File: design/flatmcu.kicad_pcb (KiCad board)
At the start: 4 copper layers, 77.8 x 63.2 mm, 127 parts, among them J1 Hall, J10 VBUS, J11 GND, J2 USB_B_Micro, J3 Throttle, J4 Motor_Phase_A, J5 Motor_Phase_B, J6 Motor_Phase_C, J7 SW Debug, J8 UART to HBD, J9 UART to BMS, Q1 TPW4R50ANH, Q2 TPW4R50ANH, Q3 TPW4R50ANH, Q4 TPW4R50ANH, Q5 TPW4R50ANH, Q6 TPW4R50ANH, Q7 Q_NMOS_GSD, Q8 Q_NMOS_GSD, U2 AP1117-33, U3 DRV8353RS, U4 STM32G431CBTx, U5 TPS563240

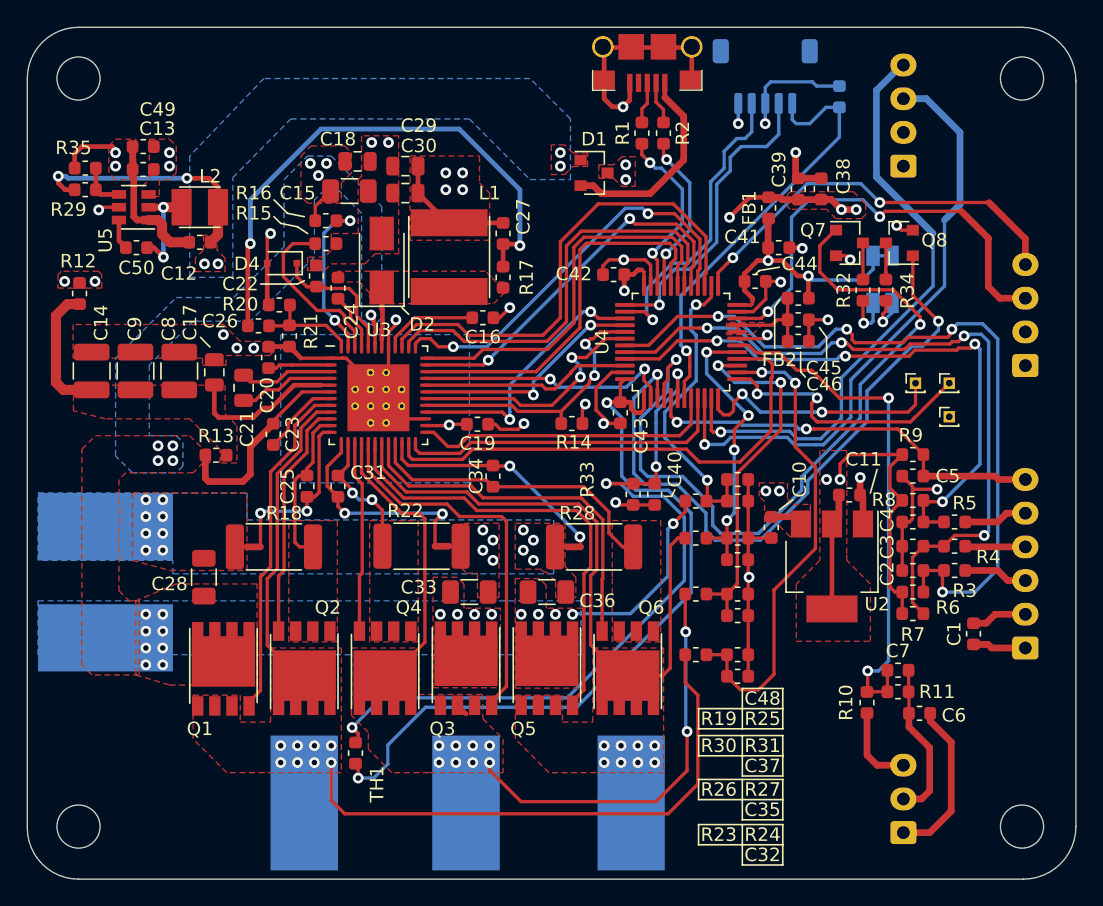
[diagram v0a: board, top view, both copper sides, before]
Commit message: updated for kicad 7
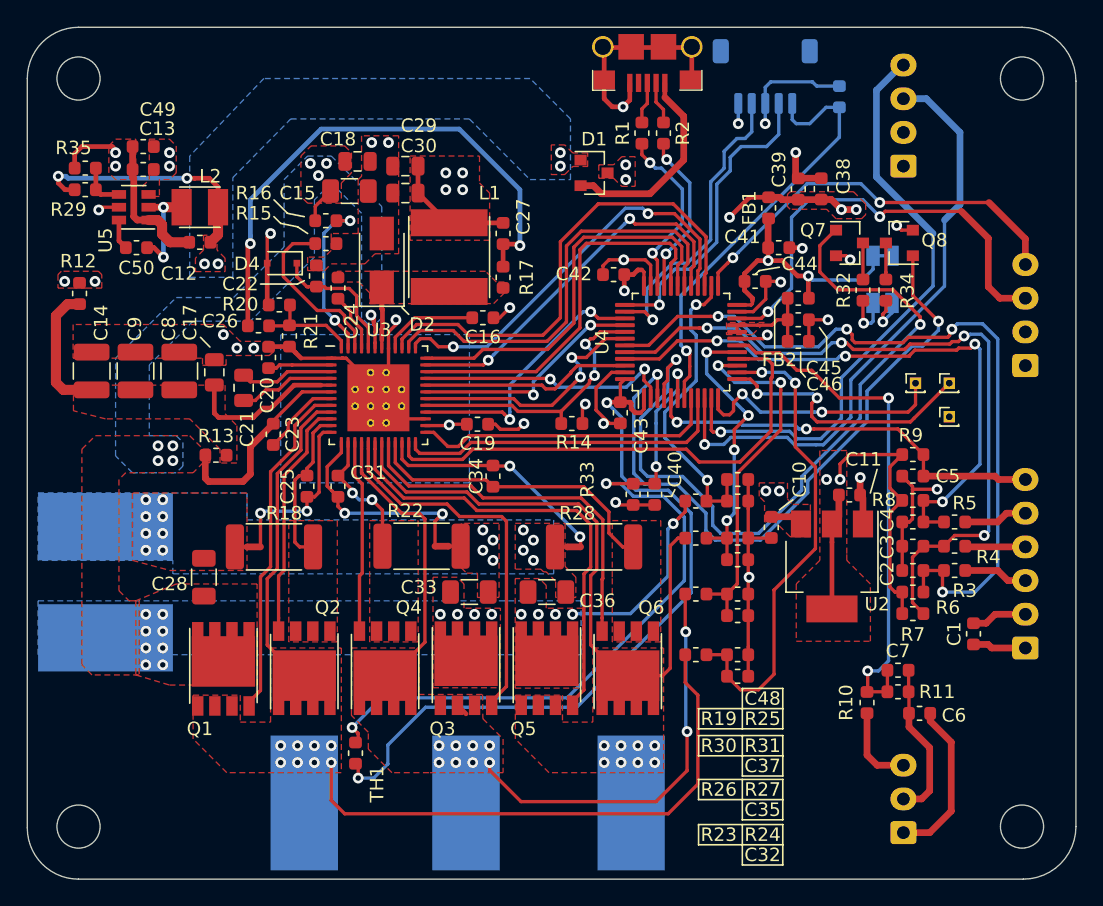
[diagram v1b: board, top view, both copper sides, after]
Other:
- net class Default removed
